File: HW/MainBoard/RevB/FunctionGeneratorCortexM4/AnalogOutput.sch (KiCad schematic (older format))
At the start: 39 parts, among them U11 LTC6910, U12 TL072, U13 TL072, U7 MCP601-xOT, U9 TS12A12511DCNR

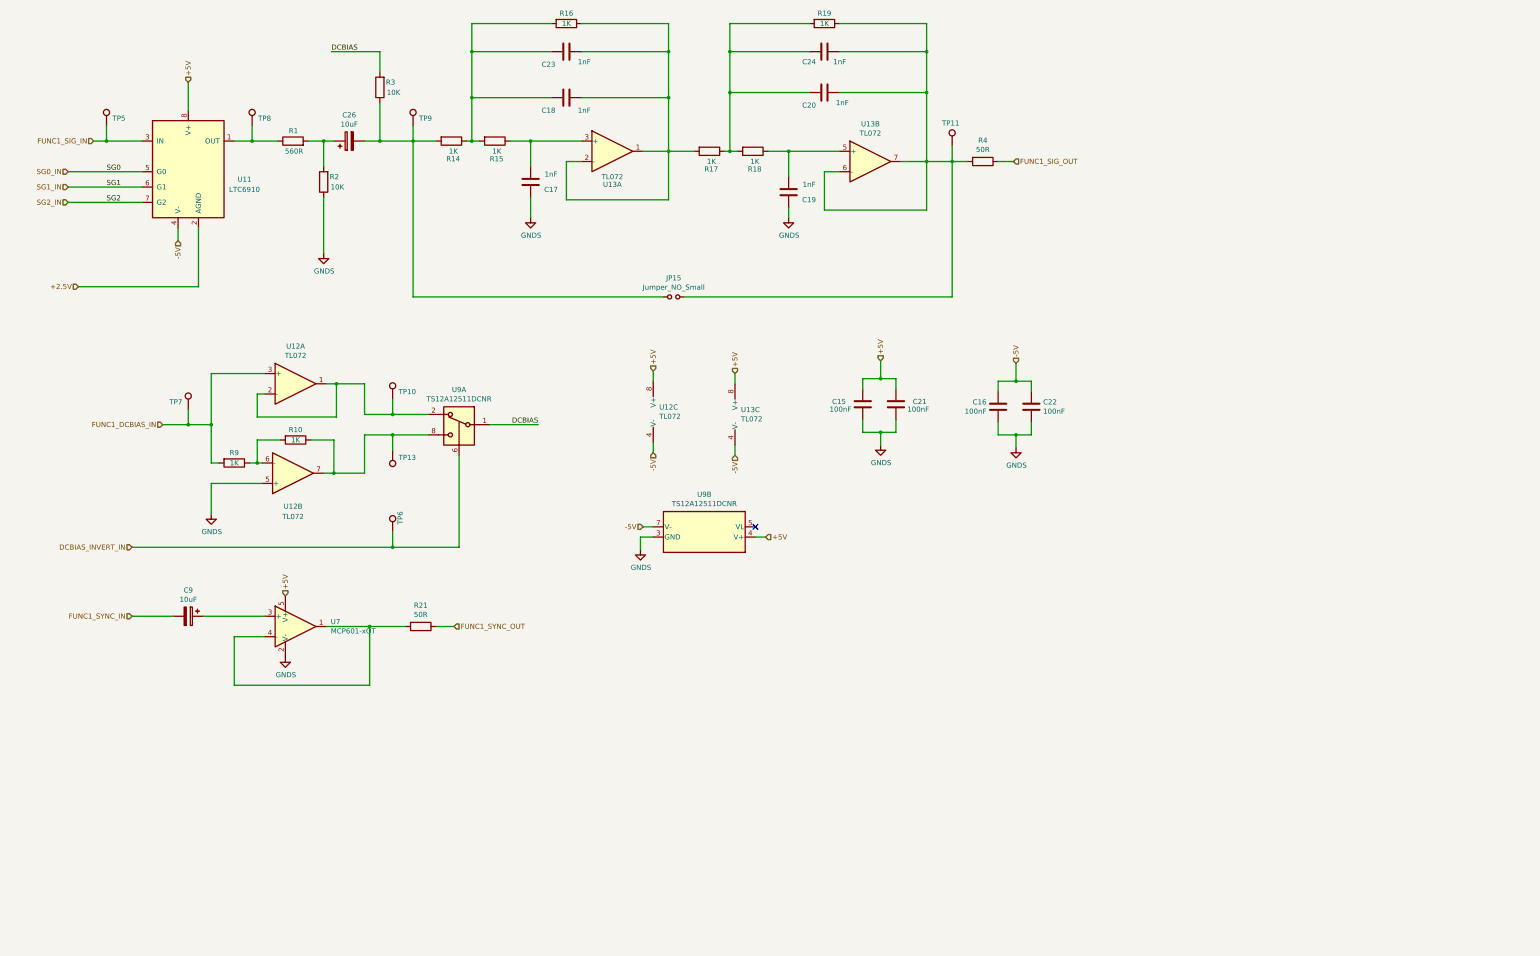
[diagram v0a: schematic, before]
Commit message: REVB DRAFT LAYOUT
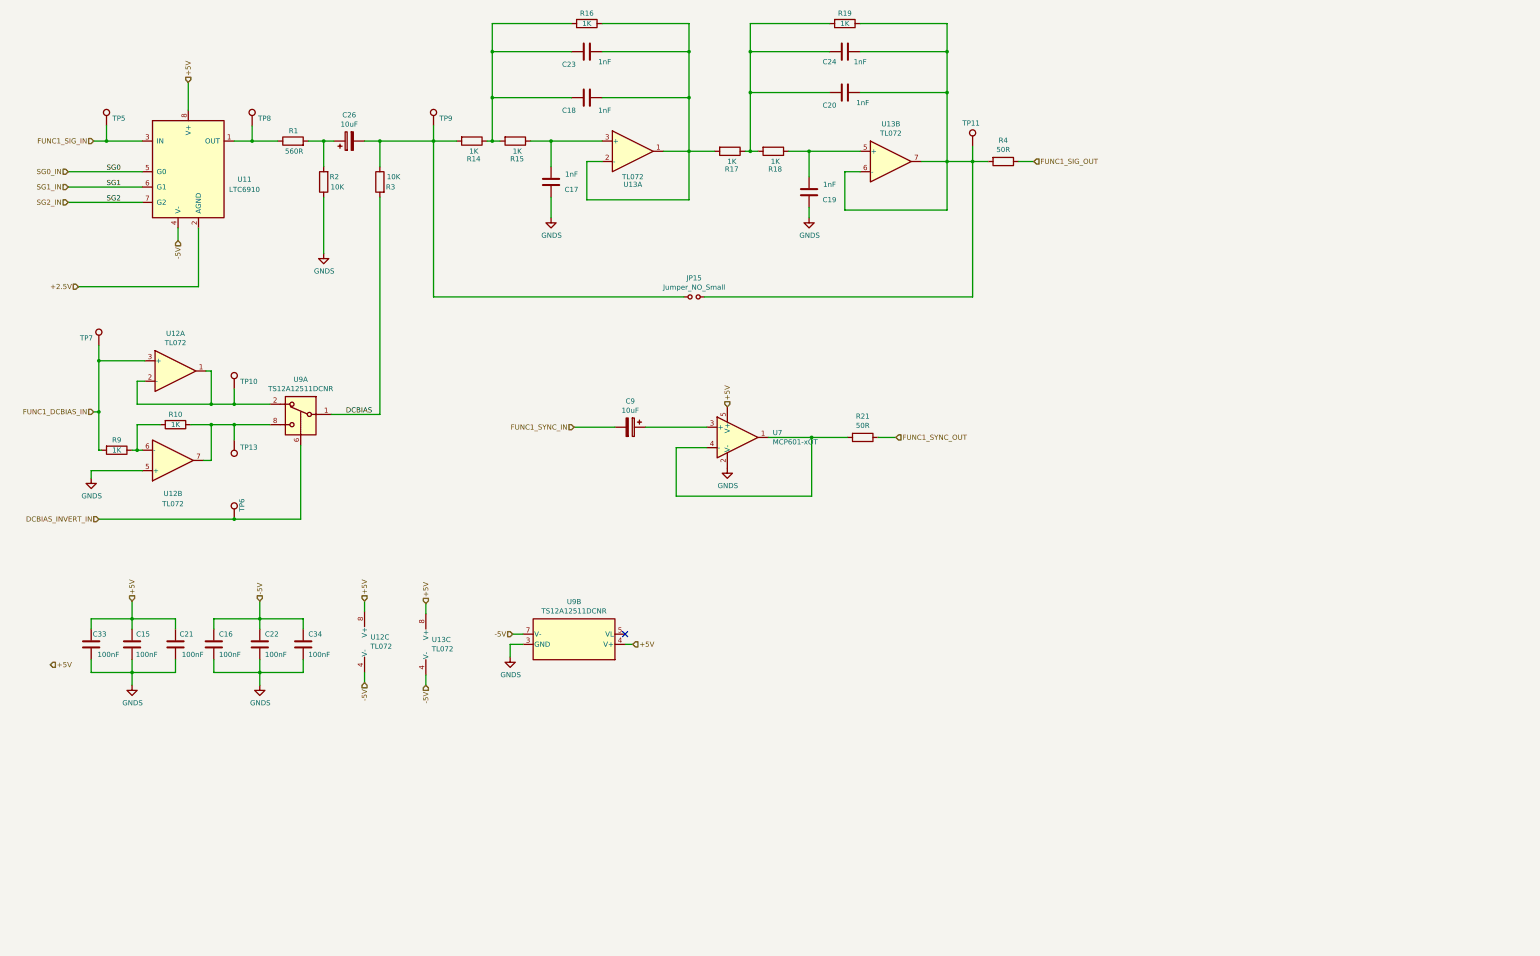
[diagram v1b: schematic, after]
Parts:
- added C33, C34: 100nF, Capacitor_SMD:C_1206_3216Metric_Pad1.42x1.75mm_HandSolder, symbol Device:C
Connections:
- net +5V: now also C33.1
- net -5V: now also C34.2
- net GNDS: now also C33.2, C34.1
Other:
- moved on the sheet: C15, C16, C17, C18, C19, C20, C21, C22, C23, C24, C9, JP15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

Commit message: OPTIMIZED REVB LAYOUT
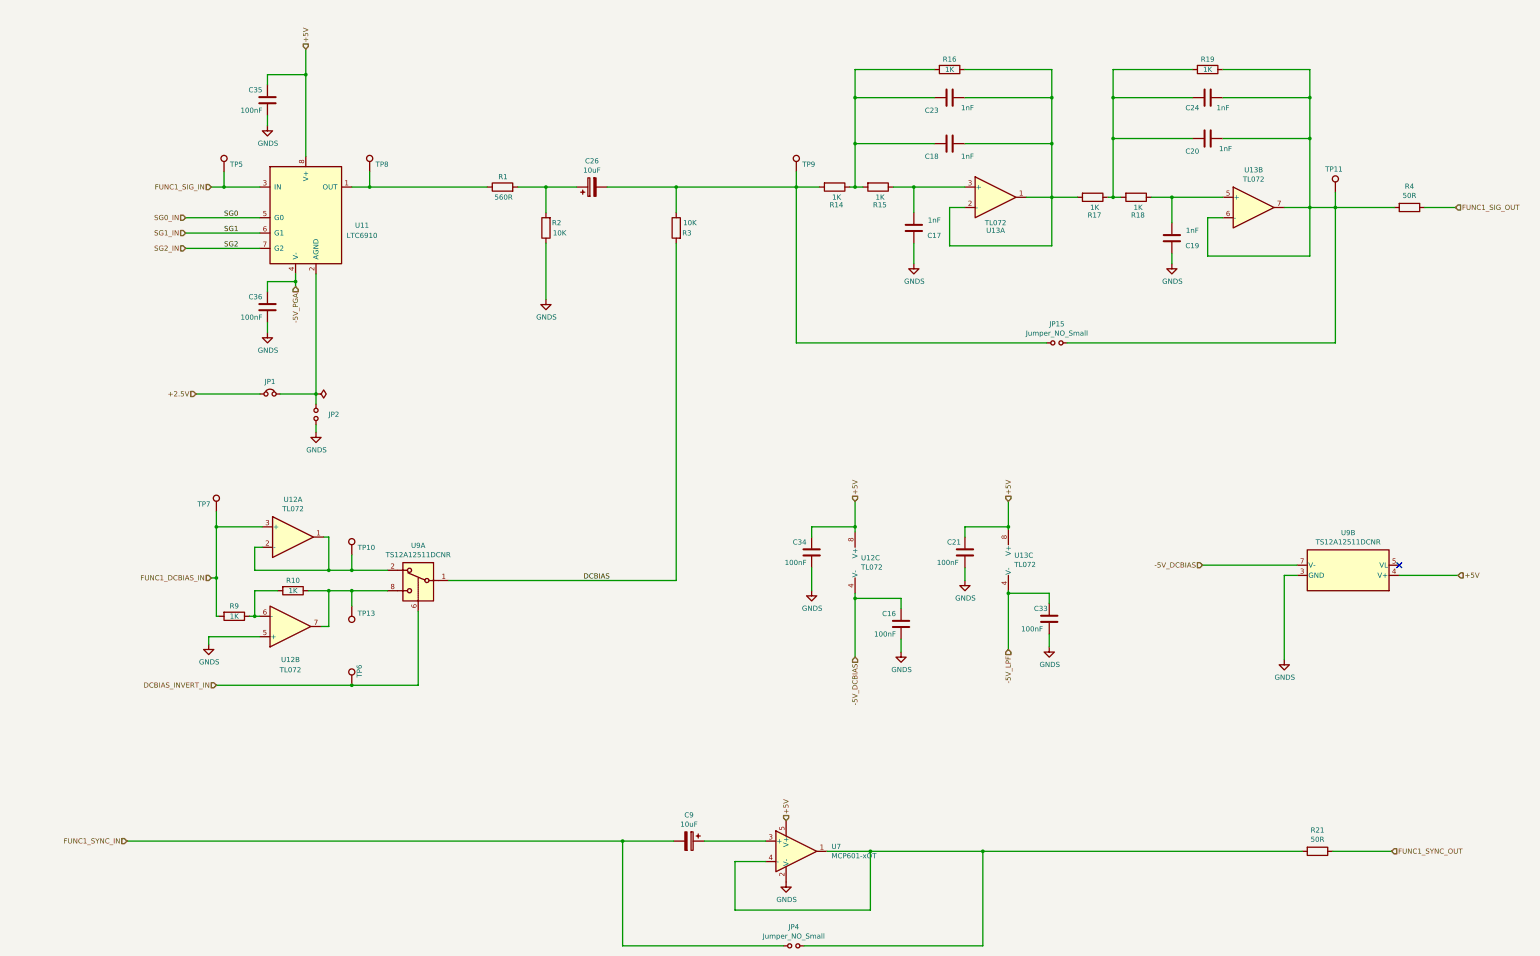
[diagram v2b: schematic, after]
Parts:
- removed C15, C22: 100nF, Capacitor_SMD:C_1206_3216Metric_Pad1.42x1.75mm_HandSolder, symbol Device:C
- added C35, C36: 100nF, Capacitor_SMD:C_1206_3216Metric_Pad1.42x1.75mm_HandSolder, symbol Device:C
- added JP1: Jumper_NC_Small, Jumper:SolderJumper-2_P1.3mm_Bridged_Pad1.0x1.5mm, symbol Device:Jumper_NC_Small
- added JP2, JP4: Jumper_NO_Small, Jumper:SolderJumper-2_P1.3mm_Open_Pad1.0x1.5mm, symbol Device:Jumper_NO_Small
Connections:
- net +2.5V: now also JP1.1; no longer U11.2 (AGND)
- net +5V: now also C34.2, C35.2; no longer C33.1
- net FUNC1_SYNC_IN: now also JP4.1
- net GNDS: now also C35.1, C36.1, JP2.2
- net at R21.2, U7.1, U7.4 (-): now also JP4.2
- net -5V renamed -5V_DCBIAS
- net -5V_DCBIAS: no longer C34.2, U11.4 (V-), U13.4 (V-)
- new net: JP1.2, JP2.1, U11.2 (AGND)
- new net -5V_LPF: C33.1, U13.4 (V-)
- new net -5V_PGA: C36.2, U11.4 (V-)
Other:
- moved on the sheet: C16, C17, C18, C19, C20, C21, C23, C24, C26, C33, C34, C9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
